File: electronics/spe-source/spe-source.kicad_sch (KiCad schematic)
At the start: 14 parts, among them J1 CONN_01X05_RA, P1 CONN_01X02

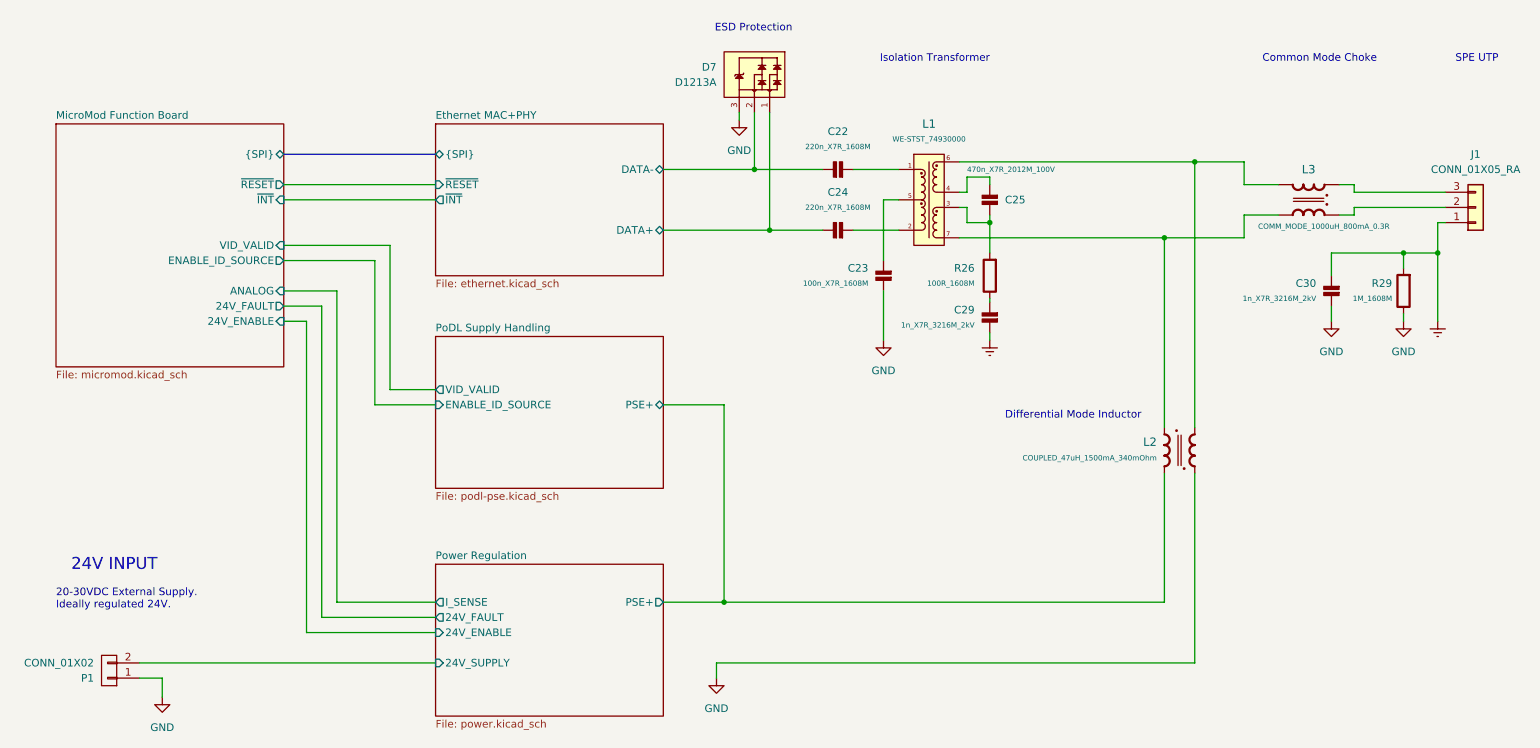
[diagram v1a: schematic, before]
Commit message: Random uncommitted KiCAD tweaks
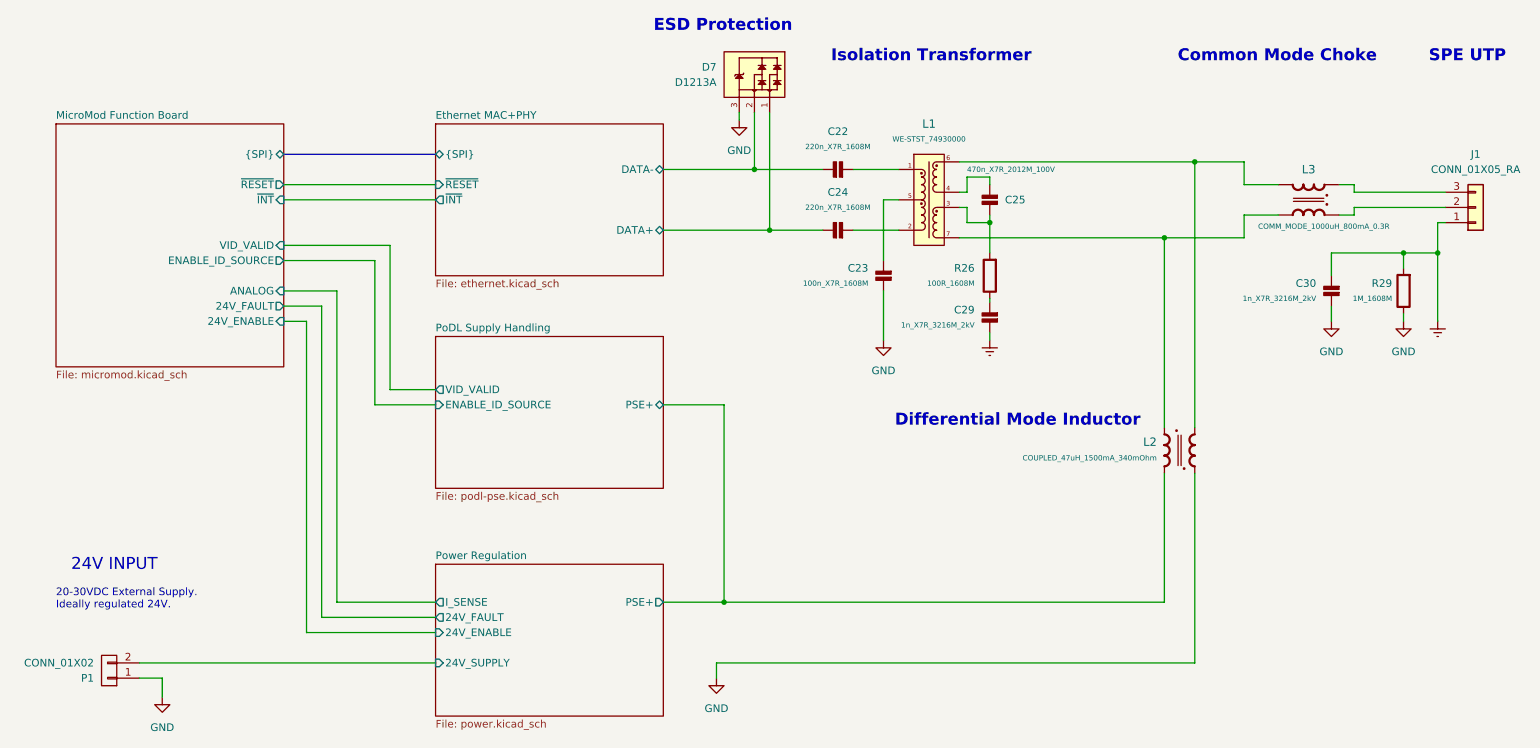
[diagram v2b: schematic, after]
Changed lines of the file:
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@@
     (comment 1 "Prototype Design")
   )
+  (bus_alias "I2C" (members "SDA" "SCL"))
   (bus_alias "SPI" (members "COPI" "CIPO" "CLK" "~{CS}"))
-  (bus_alias "I2C" (members "SDA" "SCL"))
   (junction (at 184.15 54.61) (diameter 0) (color 0 0 0 0)
   )
@@
   )
   (text "Common Mode Choke" (at 248.92 27.94 0)
-    (effects (font (size 1.27 1.27)) (justify right bottom))
+    (effects (font (size 2 2) (thickness 0.4) bold) (justify right bottom))
   )
   (text "24V INPUT" (at 30.48 113.03 0)
     (effects (font (size 2 2)) (justify left bottom))
   )
-  (text "Differential Mode Inductor" (at 186.69 87.63 0)
-    (effects (font (size 1.27 1.27)) (justify left bottom))
+  (text "Differential Mode Inductor" (at 168.275 88.9 0)
+    (effects (font (size 2 2) (thickness 0.4) bold) (justify left bottom))
   )
   (text "ESD Protection" (at 151.13 22.86 0)
-    (effects (font (size 1.27 1.27)) (justify right bottom))
-  )
-  (text "Isolation Transformer" (at 184.15 27.94 0)
-    (effects (font (size 1.25 1.25)) (justify right bottom))
-  )
-  (text "SPE UTP" (at 269.24 27.94 0)
-    (effects (font (size 1.27 1.27)) (justify right bottom))
+    (effects (font (size 2 2) (thickness 0.4) bold) (justify right bottom))
+  )
+  (text "Isolation Transformer" (at 191.135 27.94 0)
+    (effects (font (size 2 2) (thickness 0.4) bold) (justify right bottom))
+  )
+  (text "SPE UTP" (at 270.51 27.94 0)
+    (effects (font (size 2 2) (thickness 0.4) bold) (justify right bottom))
   )
   (text "20-30VDC External Supply.\nIdeally regulated 24V." (at 27.94 119.38 0)
